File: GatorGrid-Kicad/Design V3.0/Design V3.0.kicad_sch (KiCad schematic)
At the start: 30 parts, among them J1 Battery-Connector, J2 Conn_01x20_Pin, J3 Conn_01x20_Pin, J4 Conn_01x20_Pin, J5 Conn_01x20_Pin, J6 Conn_01x03, Q3 2N3904, Q4 2N3904, SW1 SW_SPST, U1 TP4056

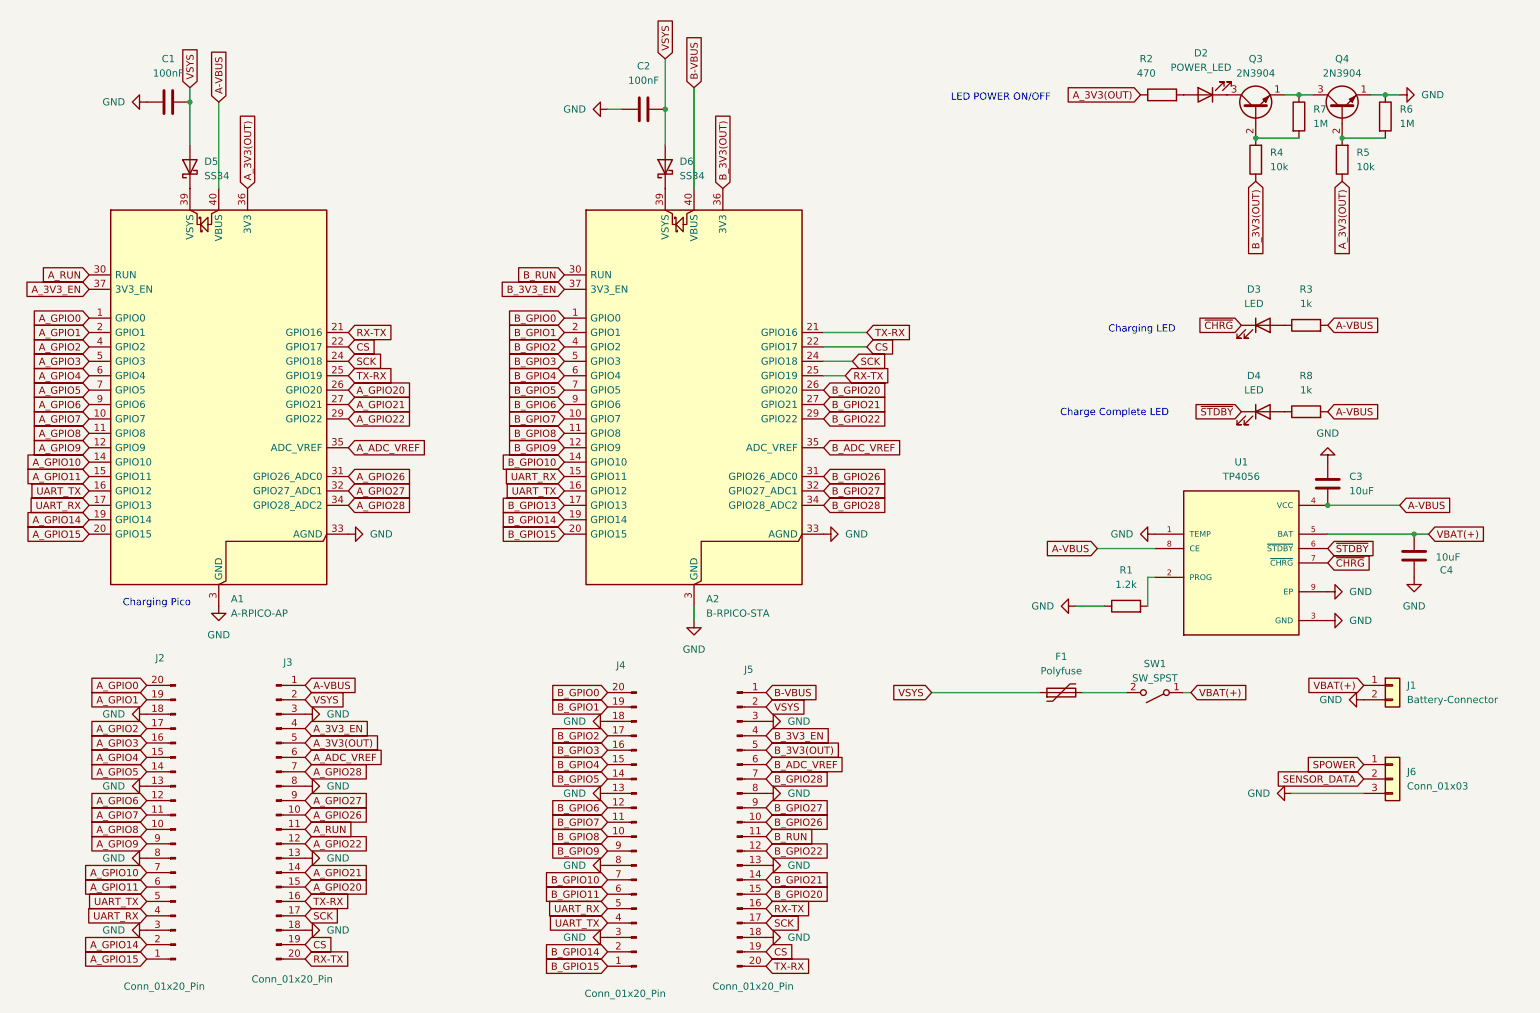
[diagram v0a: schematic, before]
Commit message: Finalized V3.0
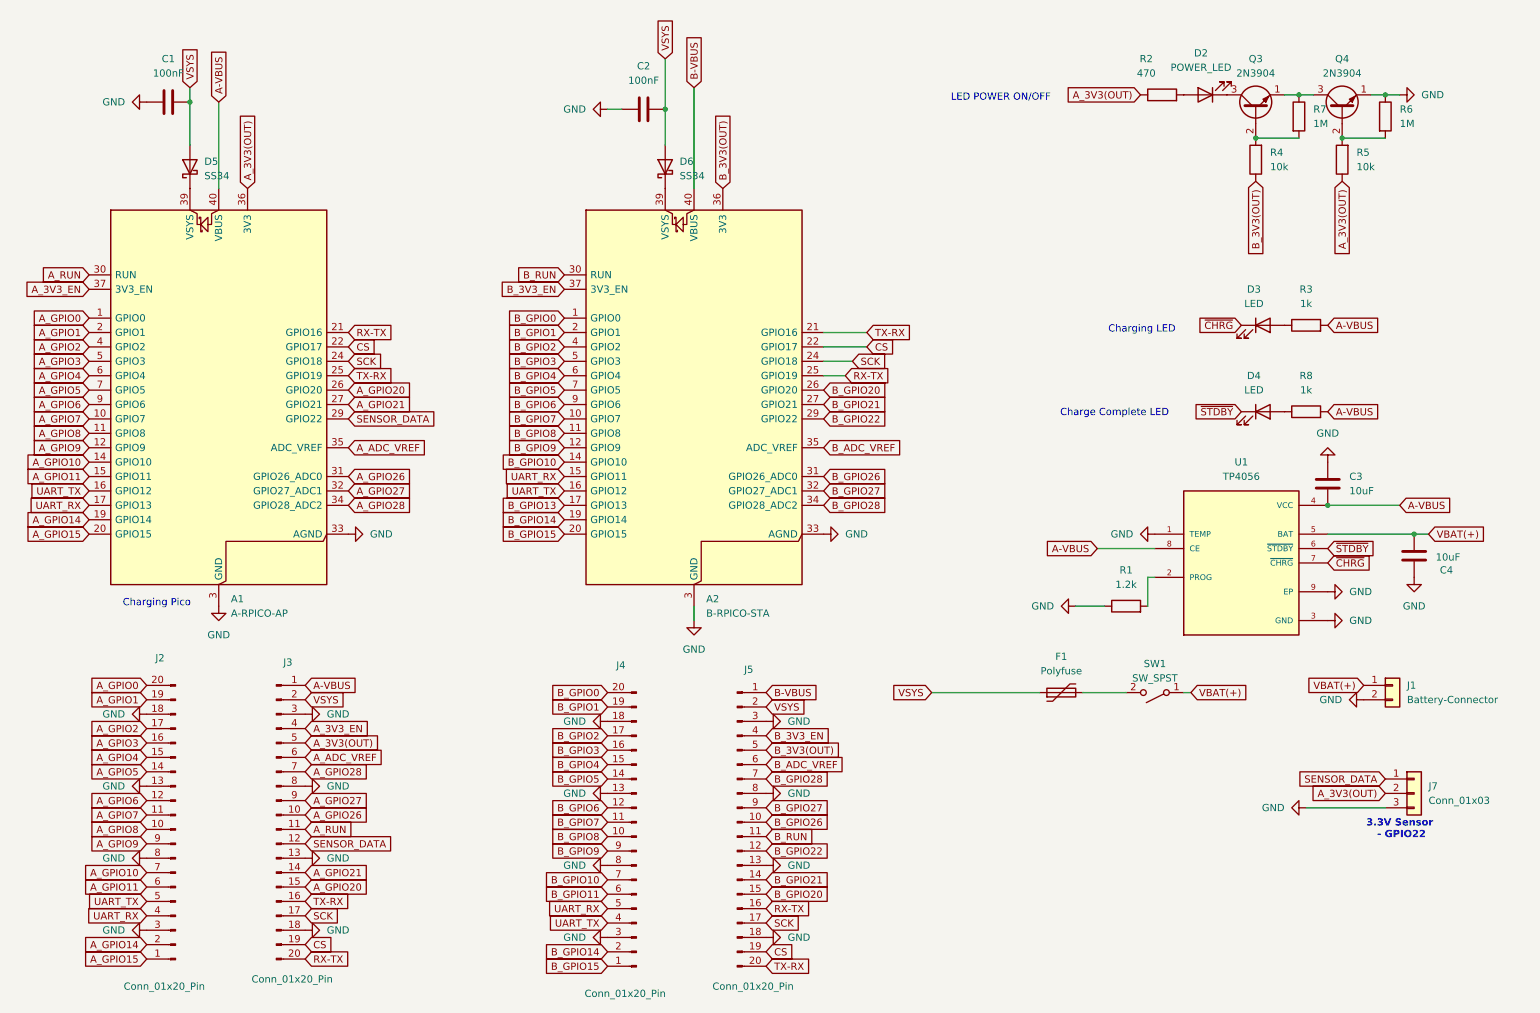
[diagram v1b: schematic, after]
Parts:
- removed J6: Conn_01x03, symbol Connector_Generic:Conn_01x03
- added J7: Conn_01x03, Connector_PinHeader_2.54mm:PinHeader_1x03_P2.54mm_Vertical, symbol Connector_Generic:Conn_01x03
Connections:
- net A_GPIO22 is gone; now on net SENSOR_DATA: A1.29 (GPIO22), J3.12 (Pin_12)
- net A_3V3(OUT): now also J7.2 (Pin_2)
- net GND: now also J7.3 (Pin_3)
- net SENSOR_DATA: now also J7.1 (Pin_1)
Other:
- note added: "3.3V Sensor - GPIO22"
